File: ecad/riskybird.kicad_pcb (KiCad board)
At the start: 2 copper layers, 58.3 x 58.3 mm, 84 parts, among them J1 USB_B_Micro, J2 Conn_01x02, J3 Conn_01x02, J4 Conn_01x02, J5 Conn_01x02, J6 Conn_01x02, J7 Conn_01x10, J8 Conn_01x10, Q1 SI2302, Q2 SI2302, Q3 SI2302, Q4 SI2302, Q5 DNBT8105-7, Q6 DNBT8105-7, Q7 Q_NMOS_GSD, SW1 SW_SPST, SW2 SW_SPST, SW3 SW_SPST, U1 MCP73831-2-OT, U10 74LVC2G08, U3 TPS2113A, U4 LP2985-3.0, U6 ESP32-C3-WROOM-02, U7 BMI088, U8 FT231XS

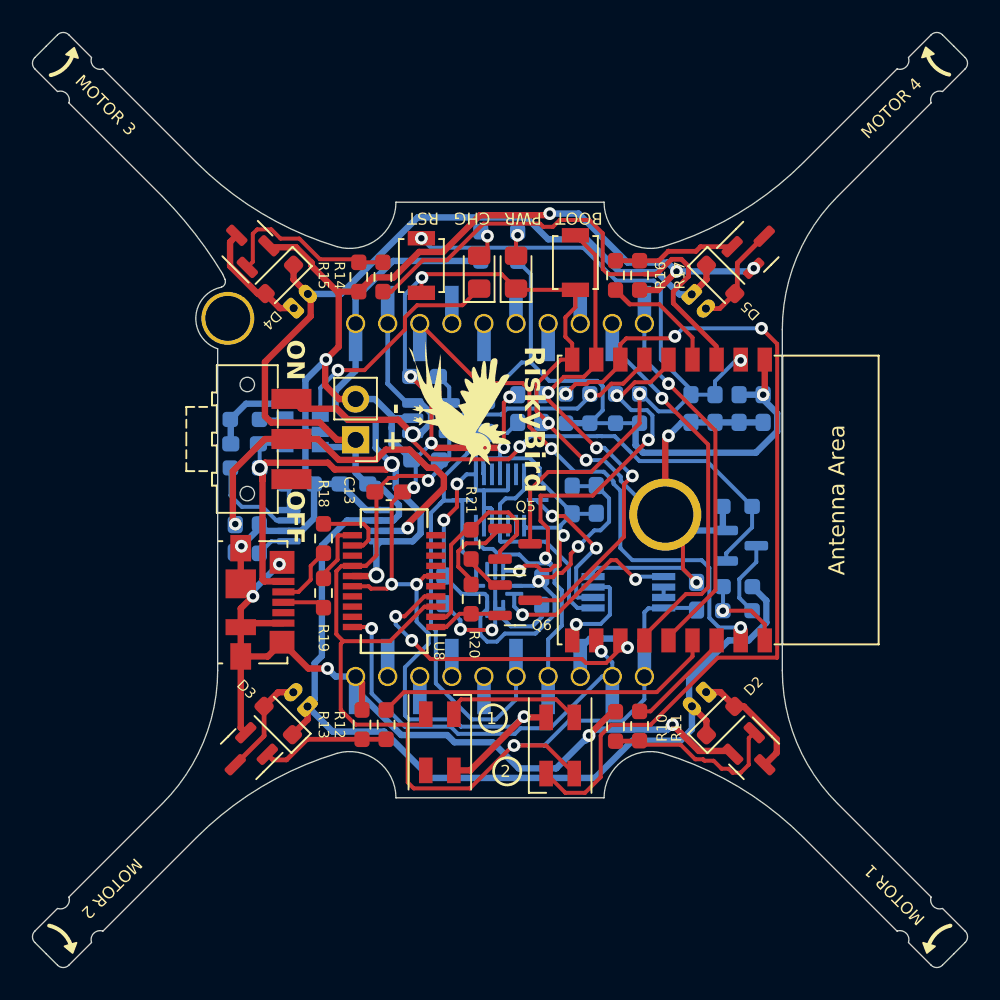
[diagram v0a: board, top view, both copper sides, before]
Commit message: RiskyBird 0.1
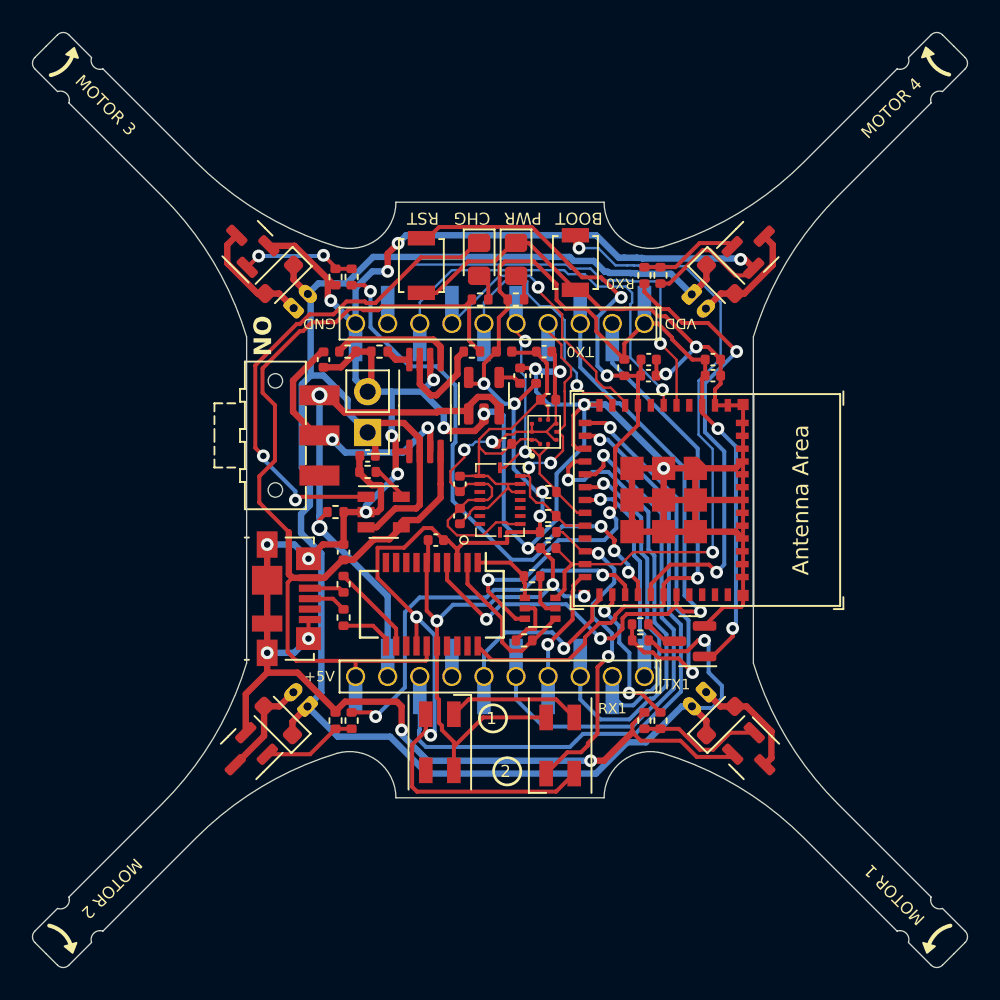
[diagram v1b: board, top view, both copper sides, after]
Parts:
- removed C14, C15, C7: 0.1u, Capacitor_SMD:C_0603_1608Metric_Pad1.08x0.95mm_HandSolder
- removed C16: 10u, Capacitor_SMD:C_0603_1608Metric_Pad1.08x0.95mm_HandSolder
- removed Q5, Q6: DNBT8105-7, Package_TO_SOT_SMD:SOT-23
- removed R23: 10k, Resistor_SMD:R_0603_1608Metric_Pad0.98x0.95mm_HandSolder
- removed REF**: wire_hole, riskybird:wire_hole
- removed U10: 74LVC2G08, Package_SO:VSSOP-8_3.0x3.0mm_P0.65mm
- removed U6: ESP32-C3-WROOM-02, Espressif:ESP32-C3-WROOM-02
- added C5: 10u, Capacitor_SMD:C_0402_1005Metric, F.Cu at (113.3, 92.2)
- added C6: 0.1u, Capacitor_SMD:C_0402_1005Metric, F.Cu at (113.3, 91.2)
- added C8: 0.1u, Capacitor_SMD:C_0402_1005Metric, F.Cu at (109.2, 92.2)
- added Q8: BC847BDW1, Package_TO_SOT_SMD:SOT-363_SC-70-6, F.Cu at (102.5, 106.8)
- added R26: 10k, Resistor_SMD:R_0402_1005Metric, F.Cu at (103.0, 102.0)
- added U5: ESP32-C6-MINI-1/U, Espressif:ESP32-C6-MINI-1, F.Cu at (112.9, 100.0)
- C1, C10, C11, C12, C17, C18, C19, C2, C20, C21, C3, C4: footprint Capacitor_SMD:C_0603_1608Metric_Pad1.08x0.95mm_HandSolder -> Capacitor_SMD:C_0402_1005Metric; moved to F.Cu
- C13: footprint Capacitor_SMD:C_0603_1608Metric_Pad1.08x0.95mm_HandSolder -> Capacitor_SMD:C_0402_1005Metric
- G***, JP2: moved to B.Cu
- L1: footprint Inductor_SMD:L_0805_2012Metric_Pad1.15x1.40mm_HandSolder -> Inductor_SMD:L_0402_1005Metric; moved to F.Cu
- Q7, U1, U3, U4: moved to F.Cu
- R1, R2, R22, R24, R25, R3, R4, R5, R6, R7, R8, R9: footprint Resistor_SMD:R_0603_1608Metric_Pad0.98x0.95mm_HandSolder -> Resistor_SMD:R_0402_1005Metric; moved to F.Cu
- R10, R11, R12, R13, R14, R15, R16, R17, R18, R19, R20, R21: footprint Resistor_SMD:R_0603_1608Metric_Pad0.98x0.95mm_HandSolder -> Resistor_SMD:R_0402_1005Metric
- U2: footprint riskybird:BMP390_Handsolder -> riskybird:BMP390; moved to F.Cu
- U7: footprint riskybird:BMI088_Handsolder -> riskybird:BMI088; moved to F.Cu
- moved G*** 32.2 mm to (100.5, 84.0), turned to 0 degrees
- moved R4 25.1 mm to (89.8, 100.8), turned to 0 degrees
- moved G*** 22.1 mm to (100.2, 115.8), turned to 180 degrees
- moved J7 22.0 mm to (100.0, 89.0)
- moved J8 22.0 mm to (100.0, 111.0)
- moved R6 15.9 mm to (98.2, 90.8)
- moved G*** 13.1 mm to (100.0, 100.0)
- moved R7 12.9 mm to (90.5, 90.8), turned to 0 degrees
- moved C19 12.4 mm to (89.0, 91.2)
- moved C3 12.0 mm to (103.0, 93.8), turned to 0 degrees
- moved U2 10.3 mm to (102.8, 95.8), turned to 180 degrees
- moved C4 9.84 mm to (100.2, 96.5), turned to 180 degrees
- moved R3 9.64 mm to (92.5, 90.8), turned to 180 degrees
- moved U3 9.37 mm to (95.3, 94.1), turned to -90 degrees
- moved C1 9.14 mm to (90.2, 103.2), turned to 90 degrees
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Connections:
- J7 pad 6: unconnected-(J7-Pin_6-Pad6) -> /IO1
- J7 pad 7: unconnected-(J7-Pin_7-Pad7) -> /IO2
- J7 pad 8: unconnected-(J7-Pin_8-Pad8) -> /IO3
- J7 pad 9: unconnected-(J7-Pin_9-Pad9) -> /IO4
- J8 pad 3: unconnected-(J8-Pin_3-Pad3) -> /SCK
- J8 pad 4: unconnected-(J8-Pin_4-Pad4) -> /MISO
- J8 pad 5: unconnected-(J8-Pin_5-Pad5) -> /MOSI
- J8 pad 6: unconnected-(J8-Pin_6-Pad6) -> /IO5
- Q7 pad 1: VCOM -> VDD
- R4 pad 2: GNDD -> GND
- R8 pad 2: /SDA -> /SCL
- R9 pad 2: /SCL -> /SDA
- U2 pad 7: /INT_BARO -> unconnected-(U2-INT-Pad7)
- U7 pad 1: /INT_GYR -> unconnected-(U7-INT2-Pad1)
- U7 pad 12: /INT_GYR -> unconnected-(U7-INT3-Pad12)
- U7 pad 16: /INT_ACC -> unconnected-(U7-INT1-Pad16)
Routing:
- net GNDD: track 114.1 -> 152.6 mm, vias 11 -> 9
- net /RGB_CTRL: track 55.5 -> 20.6 mm, vias 3 -> 2
- net /MOSI: track 0.00 -> 31.3 mm, vias 0 -> 1
- net /SCL: track 46.6 -> 17.5 mm, vias 1 -> 2
- net /IO4: track 0.00 -> 28.1 mm, vias 0 -> 1
- net /SCK: track 0.00 -> 27.7 mm, vias 0 -> 1
- net /IO3: track 0.00 -> 23.9 mm, vias 0 -> 1
- net /MOTOR4: track 7.40 -> 28.8 mm, vias 0 -> 2
- net /VSENSE: track 5.47 -> 24.7 mm, vias 1 -> 2
- net VDDA: track 46.2 -> 27.7 mm, vias 4 -> 0
- net /U0TXD: track 24.5 -> 42.4 mm
- net /SDA: track 36.4 -> 18.5 mm, vias 3 -> 2
- net /IO2: track 0.00 -> 16.9 mm, vias 0 -> 1
- net Net-(D1-K): track 14.7 -> 31.1 mm, vias 1 -> 2
- net /IO1: track 0.00 -> 15.6 mm, vias 0 -> 1
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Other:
- outline, holes or cut-outs redrawn
- board text added: "IO1"
- board text added: "IO2"
- board text added: "IO3"
- board text added: "IO4"
- board text added: "IO5"
- board text added: "MISO"
- board text added: "MOSI"
- board text added: "SCK"
- board text added: "V0.1"
- board text added: "x"
- board text added: "y"
- board text removed: "OFF"
- board text removed: "RiskyBird"
- board text removed: "RiskyBird V0.0"
